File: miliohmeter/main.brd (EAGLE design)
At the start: 53.3 x 61.9 mm, 53 parts, among them IC1 LT1019S-2.5, U2 ATMEGA169P-16AU, U3 MCP6V02-E/SN

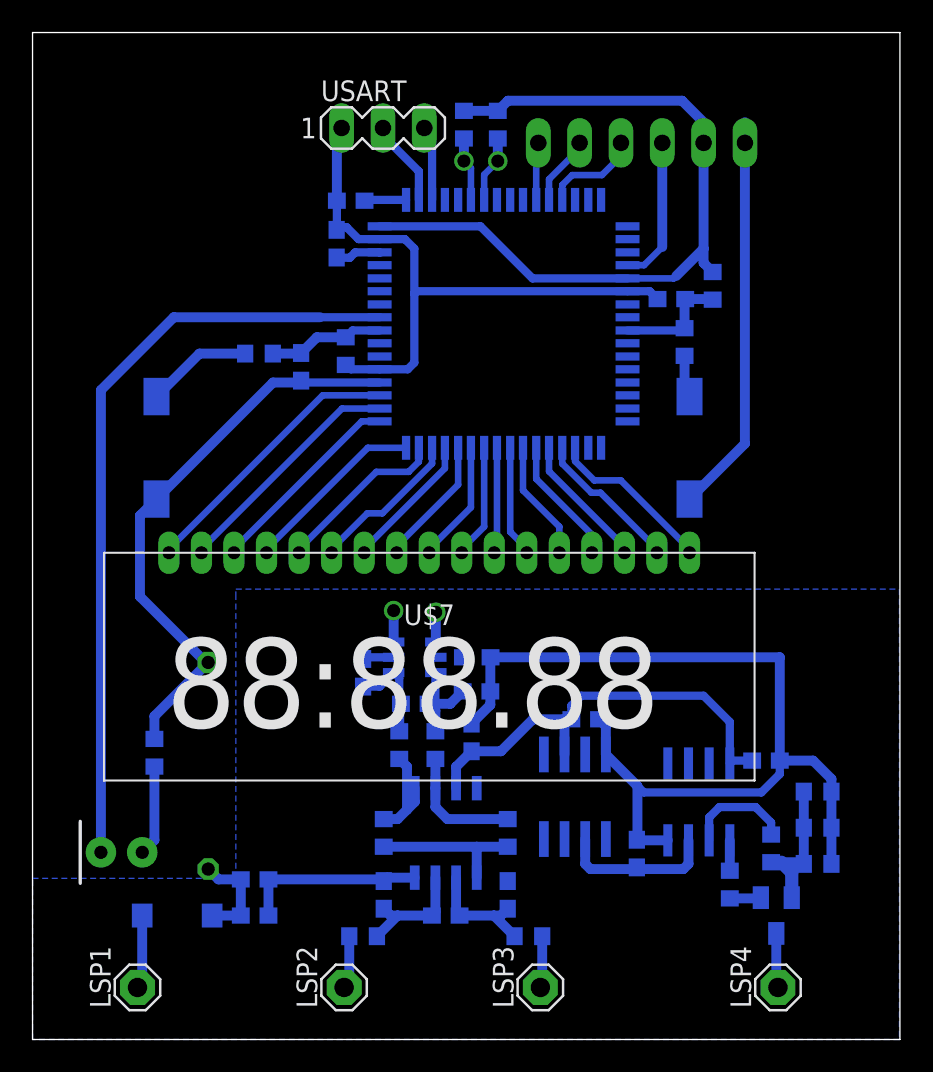
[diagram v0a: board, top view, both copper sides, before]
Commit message: updated project
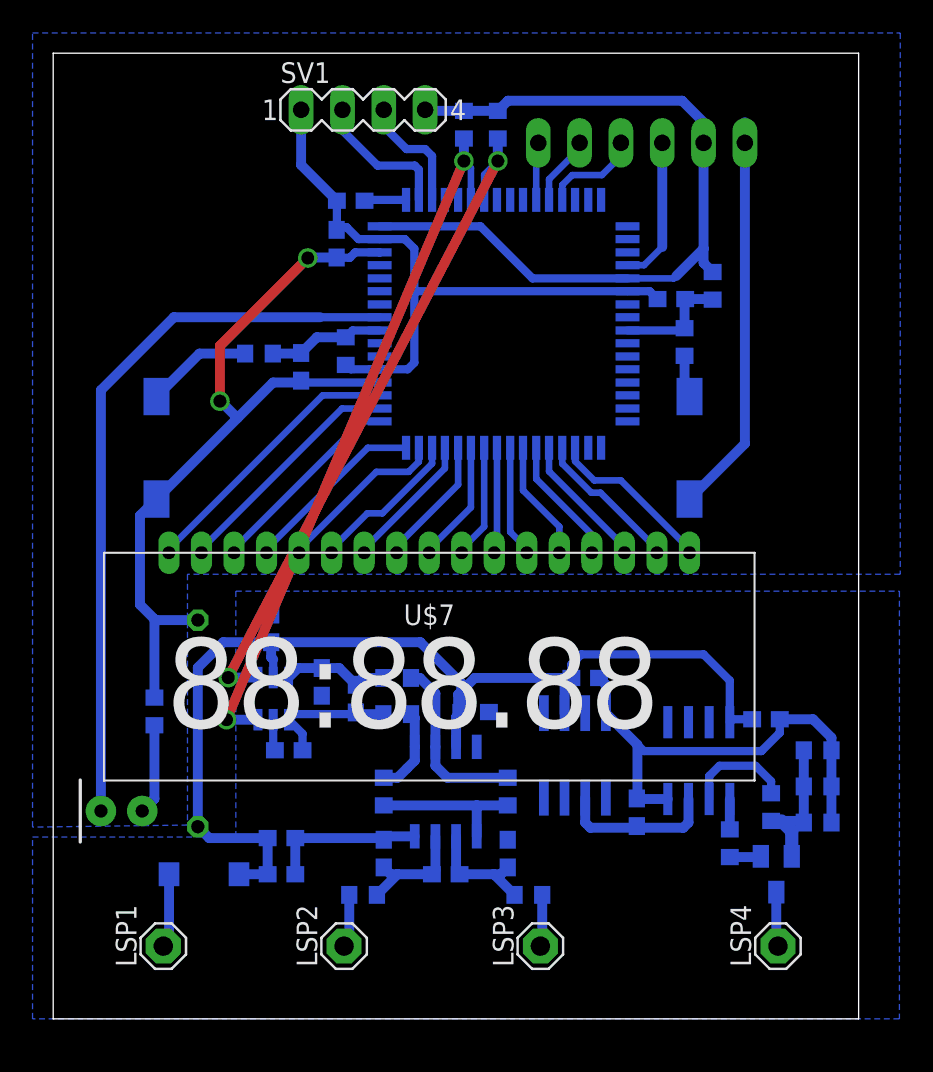
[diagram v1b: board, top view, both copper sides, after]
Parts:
- removed USART: (no value), con-lstb:MA03-1
- added SV1: (no value), con-lstb:MA04-1
- moved C10 12.8 mm to (83.2, 48.1), turned to 90 degrees
- moved C5 9.53 mm to (86.4, 44.8), turned to 270 degrees
- moved U$2 9.06 mm to (83.4, 43.8), turned to 90 degrees
- moved C6 6.60 mm to (84.3, 40.6), turned to 0 degrees
- moved R8 4.75 mm to (91.0, 45.1), turned to 180 degrees
- moved C4 3.63 mm to (88.5, 43.8), turned to 90 degrees
- moved C14 3.03 mm to (83.9, 33.0)
- moved D1 3.03 mm to (79.1, 33.0)
- moved C16 3.03 mm to (83.9, 35.2)
- moved LSP1 3.00 mm to (76.6, 28.6)
- moved R4 2.68 mm to (78.7, 42.3)
- moved C8 2.54 mm to (94.0, 33.0)
- moved T1 2.54 mm to (114.3, 33.0)
- moved C11 2.54 mm to (113.7, 42.5)
- moved C15 2.54 mm to (105.7, 36.8)
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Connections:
- removed net (TOSC1)_XTAL1: U2.24
- removed net (TOSC2)_XTAL2: U2.23
- net GND: now also SV1.1; no longer USART.1
- net RX: now also SV1.2; no longer USART.2
- net TX: now also SV1.3; no longer USART.3
- net VCC: now also SV1.4
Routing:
- net SCL: track 6.15 -> 43.5 mm
- net VCCA: track 33.5 -> 69.4 mm
- net SDA: track 5.95 -> 41.8 mm
- net GNDA: track 71.6 -> 41.2 mm
- net VCC: track 85.0 -> 99.1 mm, vias 0 -> 2
- net RX: track 5.33 -> 8.82 mm
- net VOUT: track 7.71 -> 11.1 mm
- net TX: track 4.62 -> 7.44 mm
- net LED: track 47.4 -> 44.9 mm
- net ADCIN+: track 6.35 -> 8.57 mm
- net VREF: track 6.50 -> 5.29 mm
- net GND: track 64.2 -> 64.9 mm
- added copper zone on layer 16, net GND
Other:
- board size 53.3 x 61.9 mm -> 49.5 x 59.4 mm
